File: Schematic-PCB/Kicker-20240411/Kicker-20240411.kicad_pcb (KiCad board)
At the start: 2 copper layers, 90.8 x 64.3 mm, 24 parts, among them J1 Conn_01x02_Pin, J2 Conn_01x05_Pin, J3 Conn_01x02_Pin, Q1 NMOS, Q2 NMOS, U1 TSSP58P38, U2 TSSP58P38

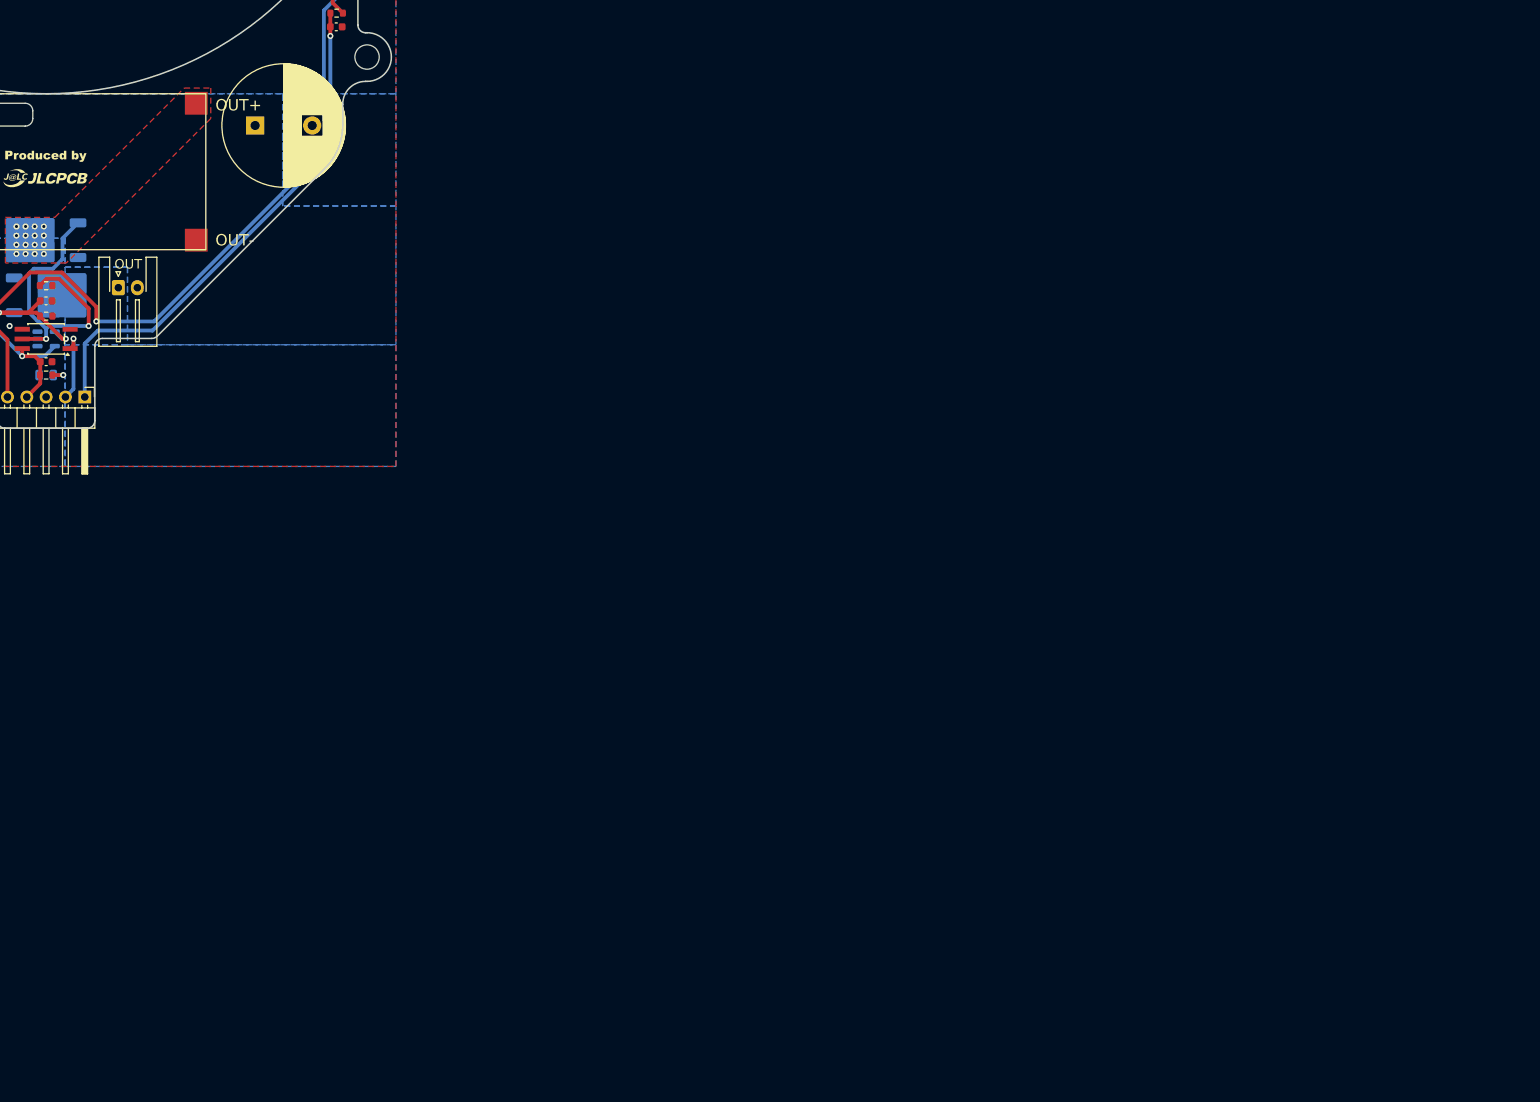
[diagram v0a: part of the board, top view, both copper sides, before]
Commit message: コミット。
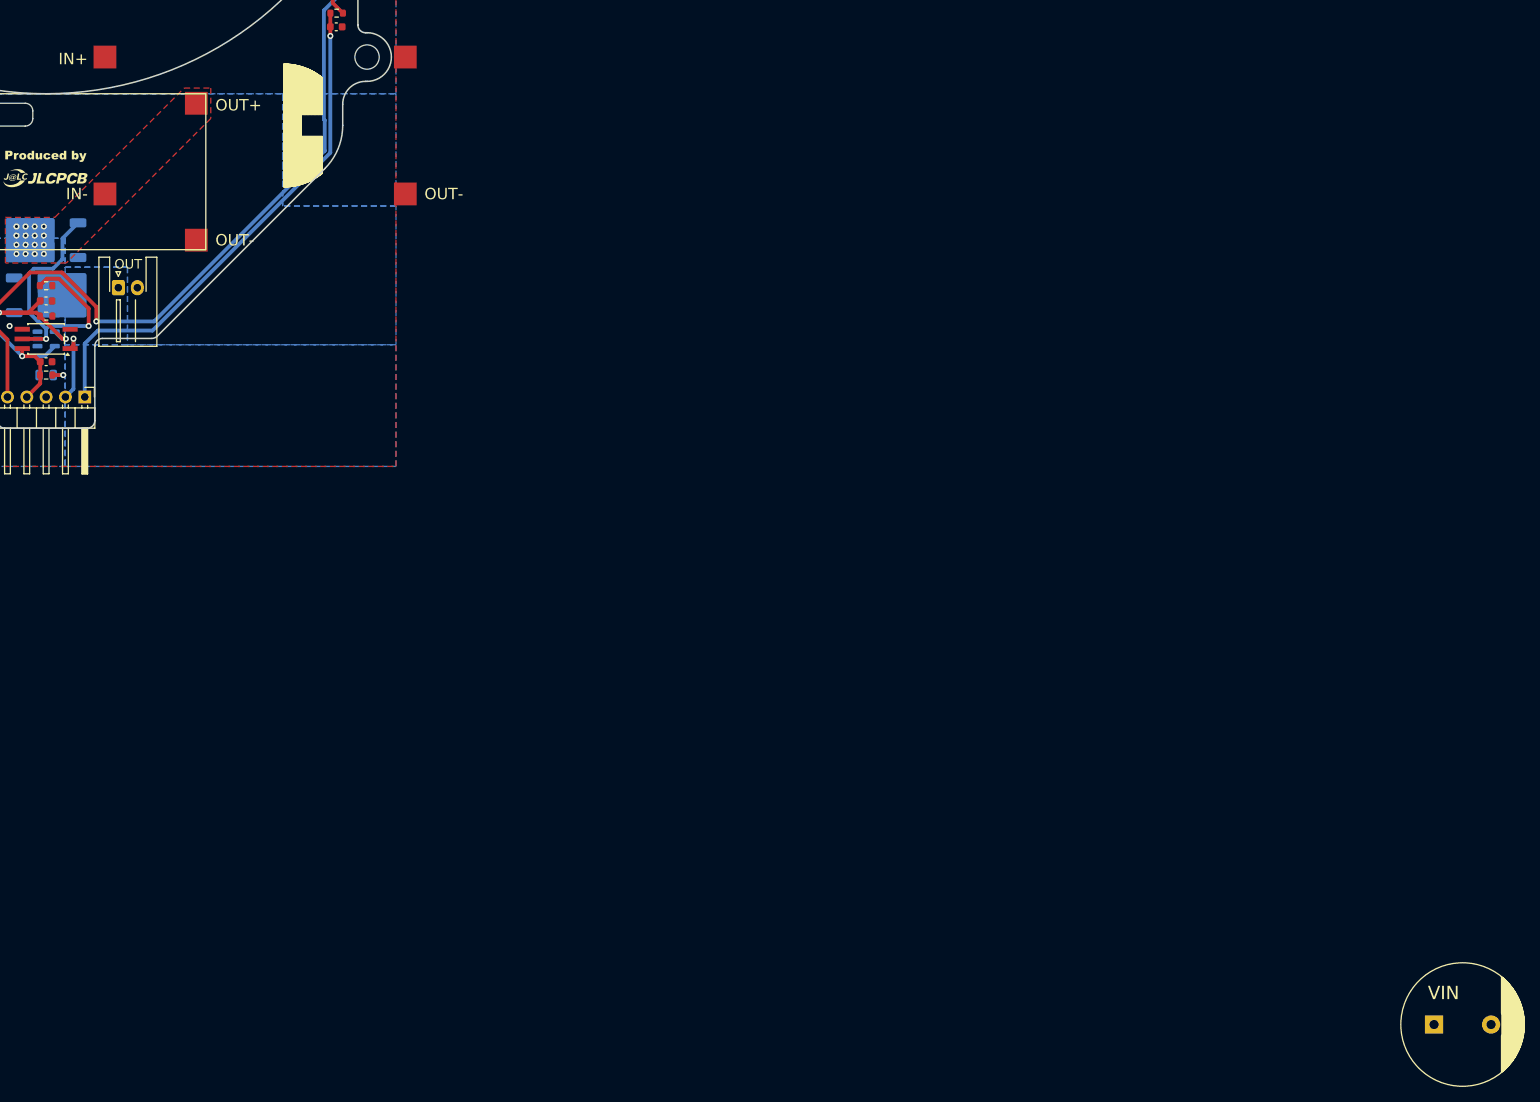
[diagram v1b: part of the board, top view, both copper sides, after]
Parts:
- added VIN: Conn_01x02_Pin, Connector_JST:JST_XH_S2B-XH-A-1_1x02_P2.50mm_Horizontal, F.Cu at (182.5, 121.7)
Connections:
- C1 pad 1: VDD -> VCC
